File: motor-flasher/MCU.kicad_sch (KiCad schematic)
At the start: 30 parts, among them J2 Conn_01x05_Pin, SW5 SS12D07VG4NSGAPA, U10 STM32F405RGT6, U8 STM32F407VGT6, Y1 CSTNE16M0V530000R0

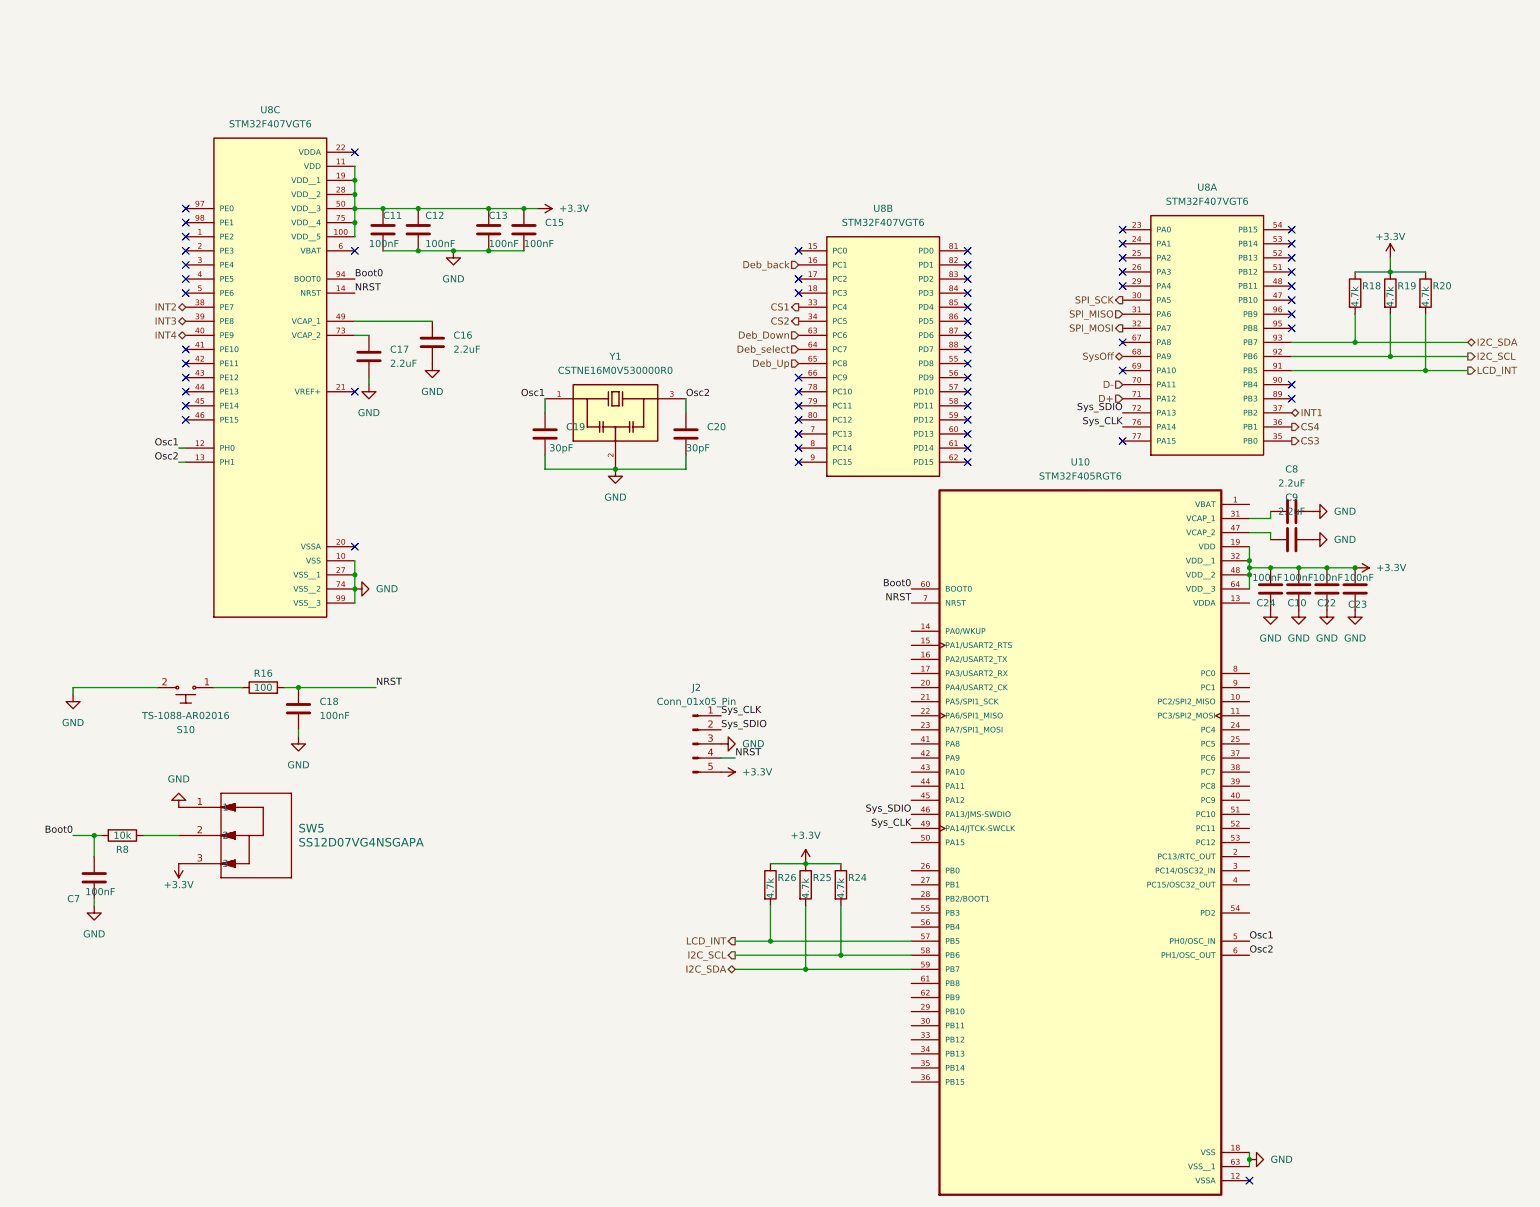
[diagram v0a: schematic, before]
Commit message: Beginning Layout Process
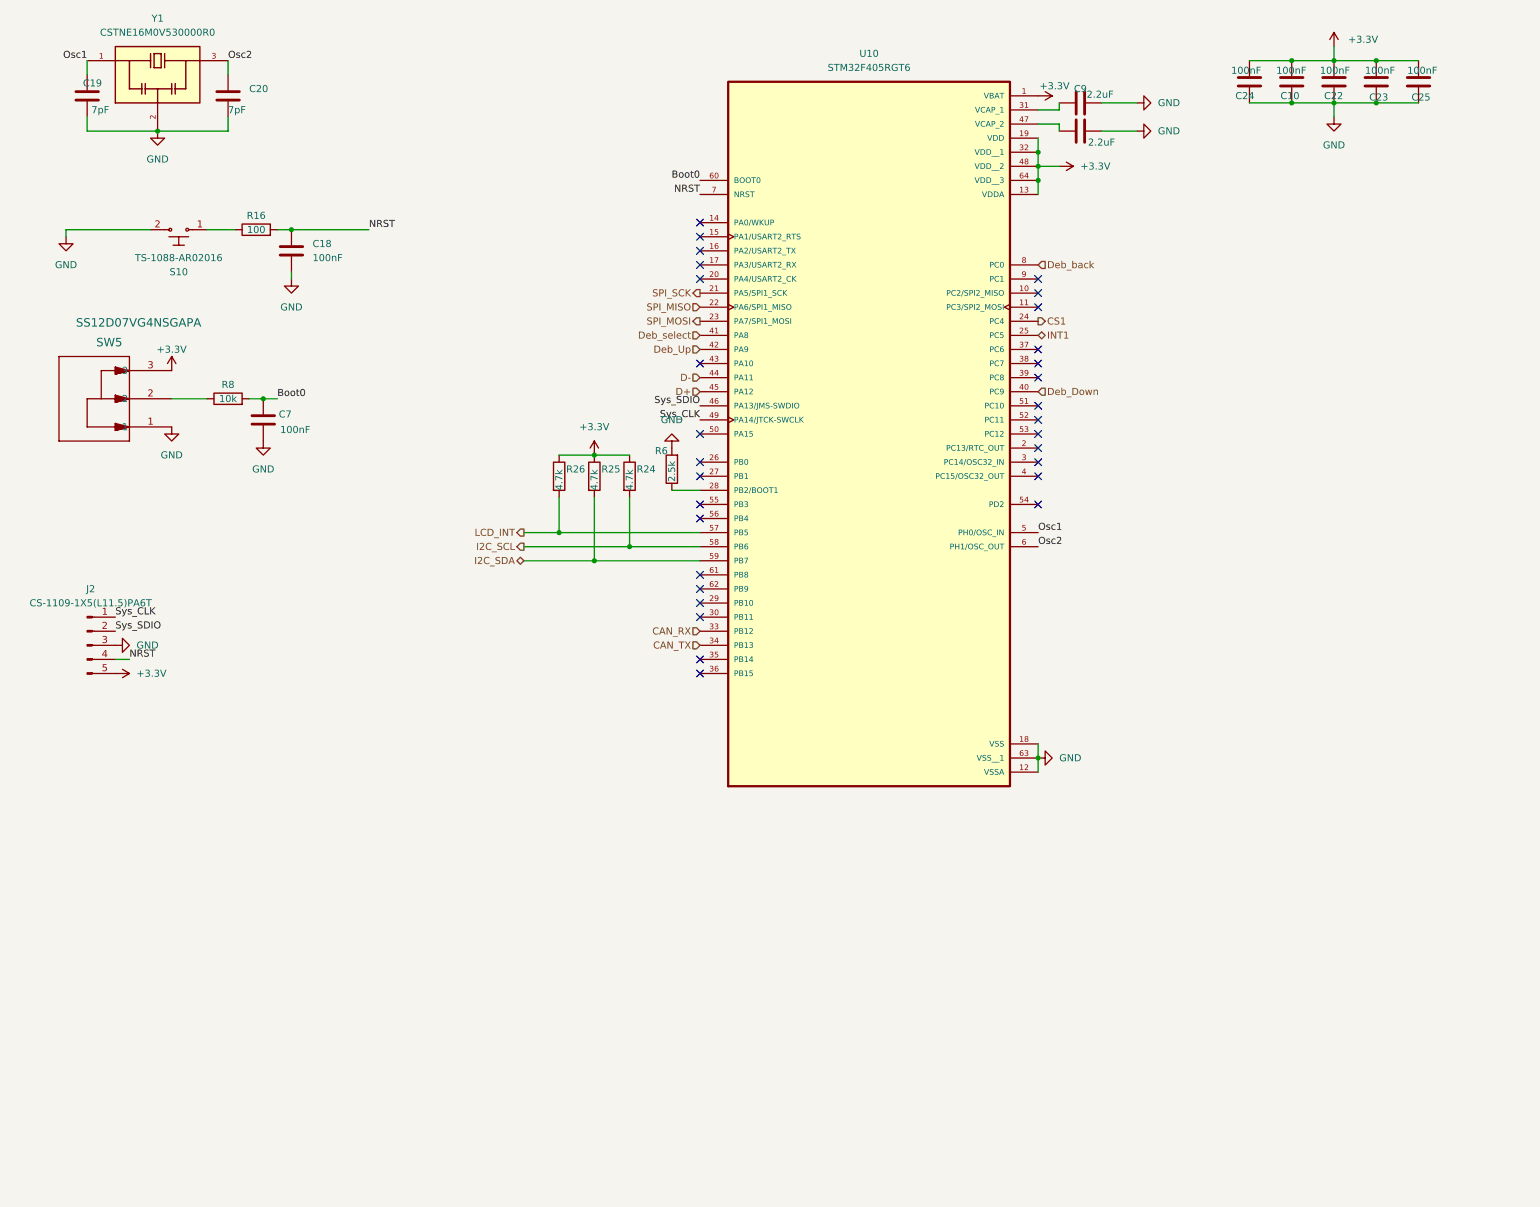
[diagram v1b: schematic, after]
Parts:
- removed C11, C12, C13, C15: 100nF, Capacitor_SMD:C_0402_1005Metric, symbol Device:C
- removed C16, C17: 2.2uF, Capacitor_SMD:C_0402_1005Metric, symbol Device:C
- removed R18, R19, R20: 4.7k, Resistor_SMD:R_0402_1005Metric, symbol Device:R
- removed U8: STM32F407VGT6, revparts2:QFP50P1600X1600X160-100N, symbol STM32F407VGT6:STM32F407VGT6
- added C25: 100nF, Capacitor_SMD:C_0402_1005Metric, symbol Device:C
- added R6: 2.5k, Resistor_SMD:R_0603_1608Metric, symbol Device:R
- C10, C22, C23, C24: footprint (none) -> Capacitor_SMD:C_0402_1005Metric
- C19, C20: value 30pF -> 7pF
- J2: value Conn_01x05_Pin -> CS-1109-1X5(L11.5)PA6T; footprint (none) -> Connector_PinHeader_2.54mm:PinHeader_1x05_P2.54mm_Horizontal
- S10: footprint revparts2:TS-1088-AR02016 -> Motor-Flasher:TS-1088-AR02016
- SW5: footprint revparts2:SS12D07_CNK -> Motor-Flasher:SOT95P275X110-6N
- U10: footprint STM32F405RGT6:QFP50P1200X1200X160-64N -> Motor-Flasher:QFP50P1200X1200X160-64N
- Y1: footprint RevParts:OSC_CSTNE16M0V530000R0 -> Motor-Flasher:OSC_CSTNE16M0V530000R0
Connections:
- net +3.3V: now also U10.1 (VBAT), U10.13 (VDDA), C25.1
- net Boot0: now also C7.1; no longer C7.2
- net CS1: now also U10.24 (PC4)
- net D+: now also U10.45 (PA12)
- net D-: now also U10.44 (PA11)
- net Deb_Down: now also U10.40 (PC9)
- net Deb_Up: now also U10.42 (PA9)
- net Deb_back: now also U10.8 (PC0)
- net Deb_select: now also U10.41 (PA8)
- net GND: now also C7.2, U10.12 (VSSA), C25.2, R6.2; no longer C7.1
- net INT1: now also U10.25 (PC5)
- net SPI_MISO: now also U10.22 (PA6/SPI1_MISO)
- net SPI_MOSI: now also U10.23 (PA7/SPI1_MOSI)
- net SPI_SCK: now also U10.21 (PA5/SPI1_SCK)
- net at U10.28 (PB2/BOOT1): now also R6.1
- net CAN_RX: now reaches U10.33 (PB12)
- net CAN_TX: now reaches U10.34 (PB13)
- no-connect marks 62 -> 30
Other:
- moved on the sheet: C10, C18, C19, C20, C22, C23, C24, C7, C9, J2, R16, R24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
